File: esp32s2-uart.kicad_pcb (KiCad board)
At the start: 2 copper layers, 30 x 14 mm, 51 parts, among them J1 USB_A, J2 USB_C_Receptacle_USB2.0, J3 Conn_02x05_Counter_Clockwise, SW1 SW_Push, U1 AMS1117-3.3, U2 USBLC6-2SC6, U3 ESP32-S2FH4, Y1 Crystal_GND24_Small

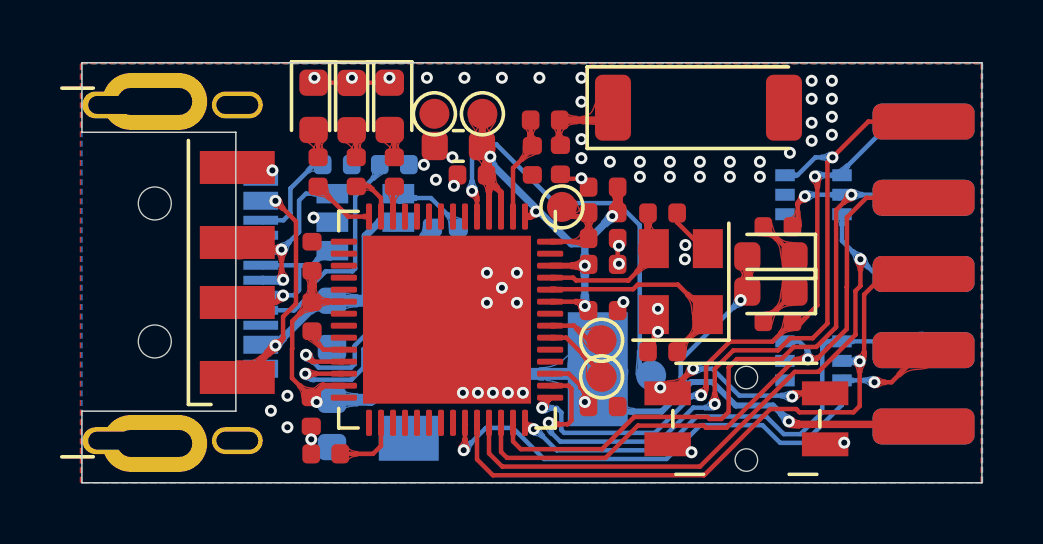
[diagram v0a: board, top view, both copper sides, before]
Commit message: v1.0
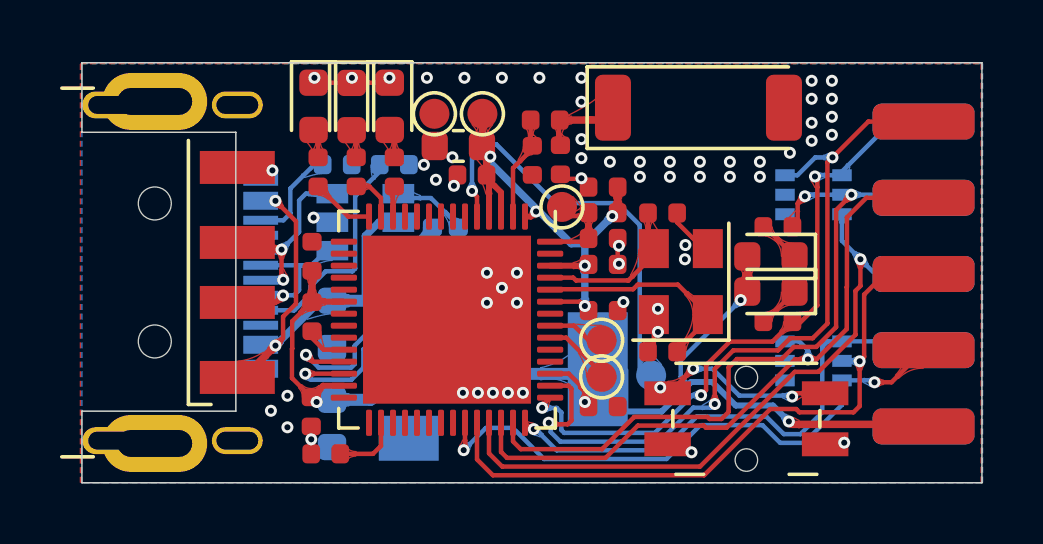
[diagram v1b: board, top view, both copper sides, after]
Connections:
- D4 pad 4: /TCK -> /IO0
- D5 pad 3: /IO0 -> /TCK
- J3 pad 1: /IO0 -> /TCK
- J3 pad 7: /TCK -> /IO0
- U3 pad 42: /TCK -> /IO0
- U3 pad 44: /IO0 -> /TCK
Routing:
- net /TCK: track 17.1 -> 25.5 mm, vias 1 -> 3
- net /IO0: track 25.5 -> 17.1 mm, vias 3 -> 1
